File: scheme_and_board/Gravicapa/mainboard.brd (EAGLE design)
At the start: 100 x 80 mm, 95 parts, among them J1 PowJack4.5, Q1 SI2301, Q2 SI2301, Q3 IRLML6402TRPBF, U1 STM32F10XRXT6LQFP64, U3 LM1117, Y1 25 MHz, Y2 8 MHz

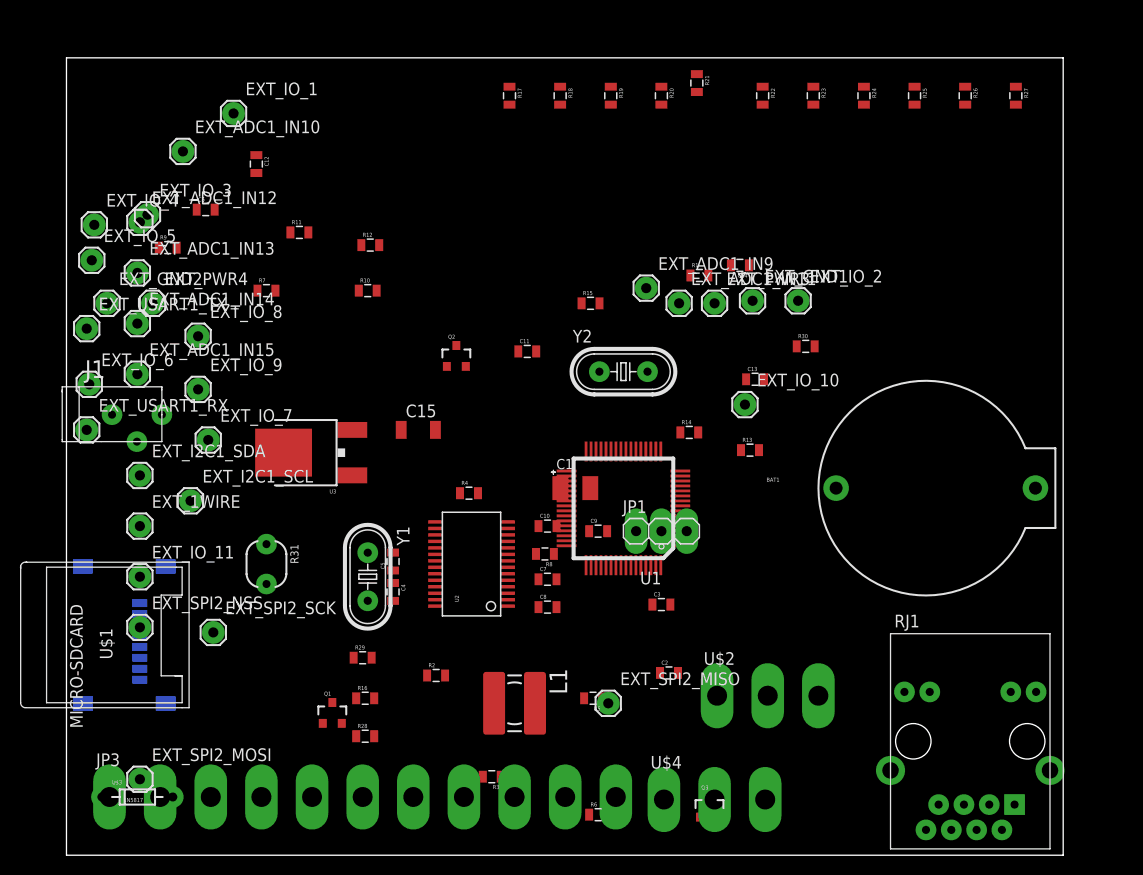
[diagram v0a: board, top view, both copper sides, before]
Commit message: eagle board
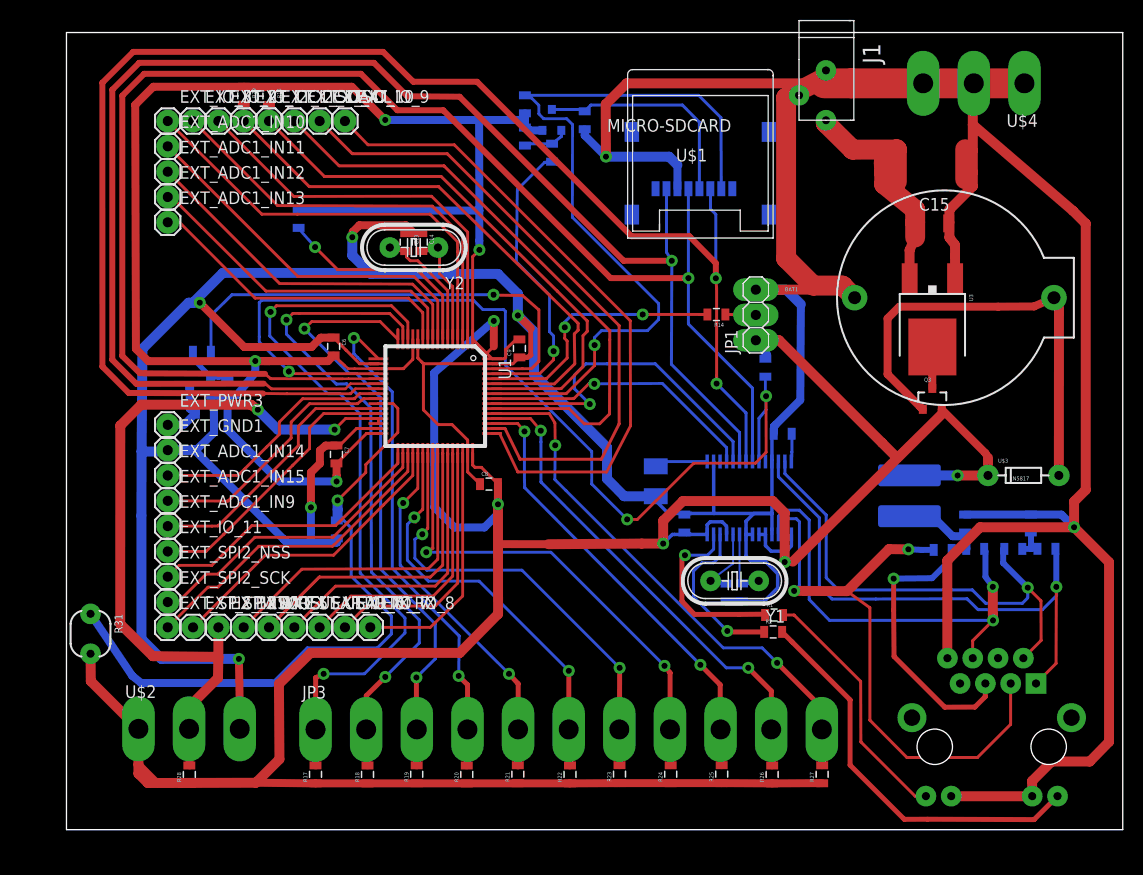
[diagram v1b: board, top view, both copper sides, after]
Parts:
- removed EXT_GND2, EXT_PWR4: (no value), GravicapaLib:1X01
- moved U$3 94.6 mm to (96.0, 38.1)
- moved J1 79.5 mm to (76.2, 78.7), turned to 180 degrees
- moved U$4 76.4 mm to (91.0, 77.4), turned to 180 degrees
- moved U$1 72.9 mm to (63.6, 67.6), turned to 180 degrees
- moved R21 71.6 mm to (45.3, 8.13), turned to 90 degrees
- moved R20 70.8 mm to (40.2, 8.10), turned to 90 degrees
- moved R17 70.8 mm to (25.0, 8.11), turned to 90 degrees
- moved R19 70.8 mm to (35.1, 8.12), turned to 90 degrees
- moved R27 70.8 mm to (75.8, 8.12), turned to 90 degrees
- moved R26 70.8 mm to (70.8, 8.10), turned to 90 degrees
- moved R23 70.8 mm to (55.5, 8.14), turned to 90 degrees
- moved R18 70.8 mm to (30.2, 8.11), turned to 90 degrees
- moved R22 70.8 mm to (50.5, 8.11), turned to 90 degrees
- moved R24 70.8 mm to (60.6, 8.13), turned to 90 degrees
- moved R25 70.8 mm to (65.7, 8.13), turned to 90 degrees
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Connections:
- net ETH_CS: now also U1.20
- net EXT_PWR: no longer EXT_PWR4.1
- net GND: no longer EXT_GND2.1
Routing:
- net GND: track 0.00 -> 562.8 mm, vias 0 -> 7
- net +3V3: track 0.00 -> 491.0 mm, vias 0 -> 9
- net SPI1_MOSI: track 0.00 -> 161.4 mm, vias 0 -> 2
- net SPI1_MISO: track 0.00 -> 151.0 mm, vias 0 -> 1
- net SPI1_SCK: track 0.00 -> 149.1 mm, vias 0 -> 1
- net ETH_CS: track 0.00 -> 99.6 mm, vias 0 -> 3
- net SD_CS: track 0.00 -> 78.7 mm, vias 0 -> 1
- net ALARM_BUS0: track 0.00 -> 75.0 mm, vias 0 -> 2
- net USART3_1WIRE: track 0.00 -> 74.9 mm, vias 0 -> 2
- net TPOUT-: track 0.00 -> 66.9 mm, vias 0 -> 2
- net ALARM_BUS1: track 0.00 -> 66.8 mm, vias 0 -> 2
- net N$28: track 0.00 -> 66.6 mm
- net N$30: track 0.00 -> 66.0 mm, vias 0 -> 1
- net N$29: track 0.00 -> 65.3 mm
- net ALARM_BUS2: track 0.00 -> 61.9 mm, vias 0 -> 2
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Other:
- board size 100 x 80 mm -> 106 x 80 mm
